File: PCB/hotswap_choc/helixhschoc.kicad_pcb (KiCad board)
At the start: 2 copper layers, 135.2 x 94 mm, 134 parts, among them J1 MJ-4PP-9, P1 CONN_01X01, P2 CONN_01X01, P3 OLED, P4 LED, SW1 SW_PUSH, SW10 SW_PUSH, SW11 SW_PUSH, SW12 SW_PUSH, SW13 SW_PUSH, SW14 SW_PUSH, SW15 SW_PUSH, SW16 SW_PUSH, SW17 SW_PUSH, SW18 SW_PUSH, SW19 SW_PUSH, SW2 SW_PUSH, SW20 SW_PUSH, SW21 SW_PUSH, SW22 SW_PUSH, SW23 SW_PUSH, SW24 SW_PUSH, SW25 SW_PUSH, SW26 SW_PUSH, SW27 SW_PUSH, SW28 SW_PUSH, SW29 SW_PUSH, SW3 SW_PUSH, SW30 SW_PUSH, SW31 SW_PUSH, SW32 SW_PUSH, SW33 Reset, SW4 SW_PUSH, SW5 SW_PUSH, SW6 SW_PUSH, SW7 SW_PUSH, SW8 SW_PUSH, SW9 SW_PUSH, U1 ProMicro, U10 SK6812mini, U11 SK6812mini, U12 SK6812mini, U13 SK6812mini, U14 SK6812mini, U15 SK6812mini, U16 SK6812mini, U17 SK6812mini, U18 SK6812mini, U19 SK6812mini, U2 SK6812mini, U20 SK6812mini, U21 SK6812mini, U22 SK6812mini, U23 SK6812mini, U24 SK6812mini, U25 SK6812mini, U26 SK6812mini, U27 SK6812mini, U28 SK6812mini, U29 SK6812mini, U3 SK6812mini, U30 SK6812mini, U31 SK6812mini, U32 SK6812mini, U33 SK6812mini, U4 SK6812mini, U5 SK6812mini, U6 SK6812mini, U7 SK6812mini, U8 SK6812mini, U9 SK6812mini

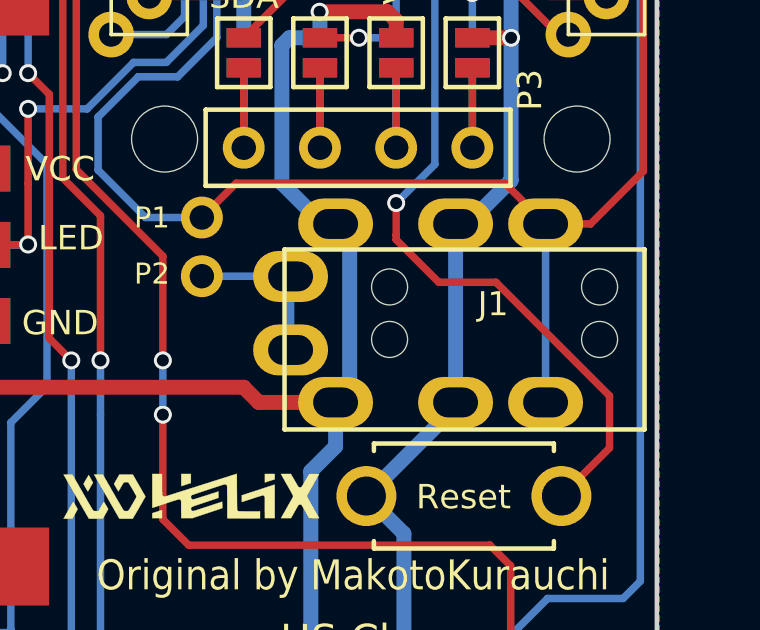
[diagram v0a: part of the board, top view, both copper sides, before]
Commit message: PCB WIP
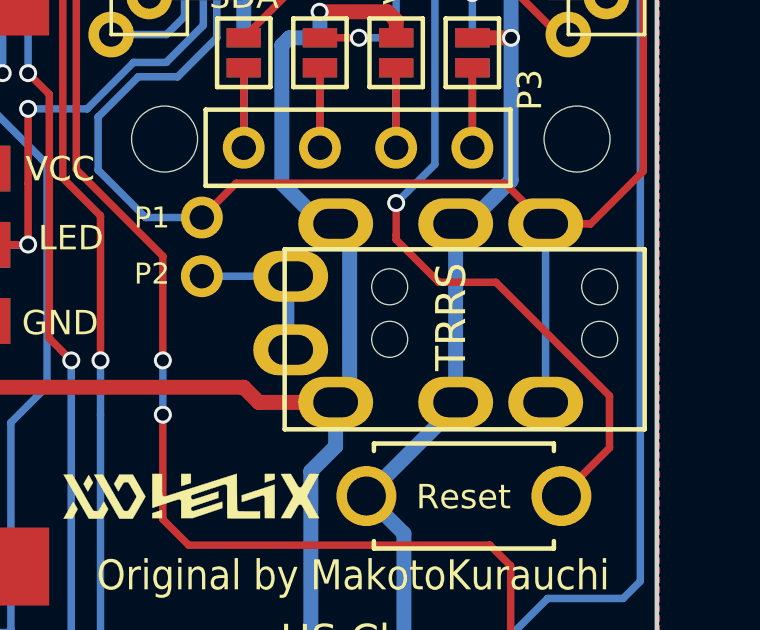
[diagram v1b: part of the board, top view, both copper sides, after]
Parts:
- J1: footprint MYLIB_REV:MJ-4PP-9_rev2 -> Random-keyboard-parts:MJ-4PP-9

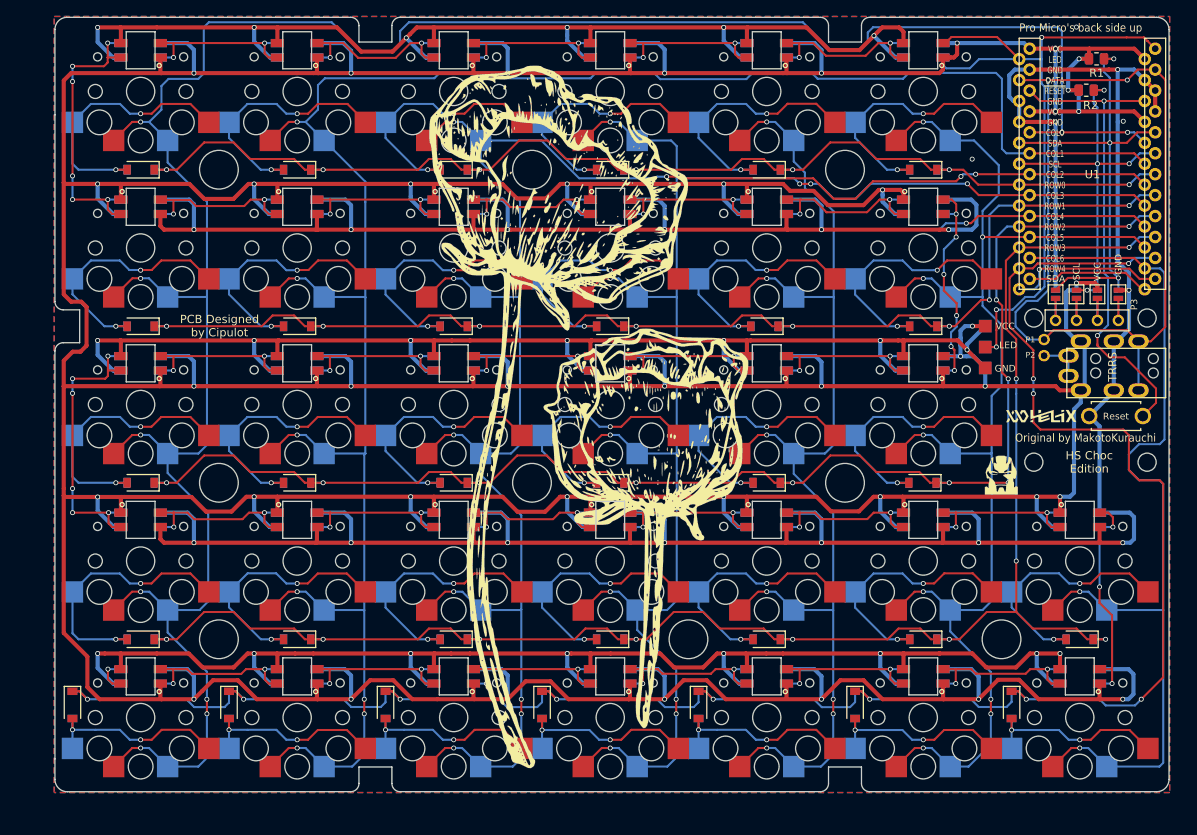
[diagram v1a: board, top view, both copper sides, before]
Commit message: PCB WIP
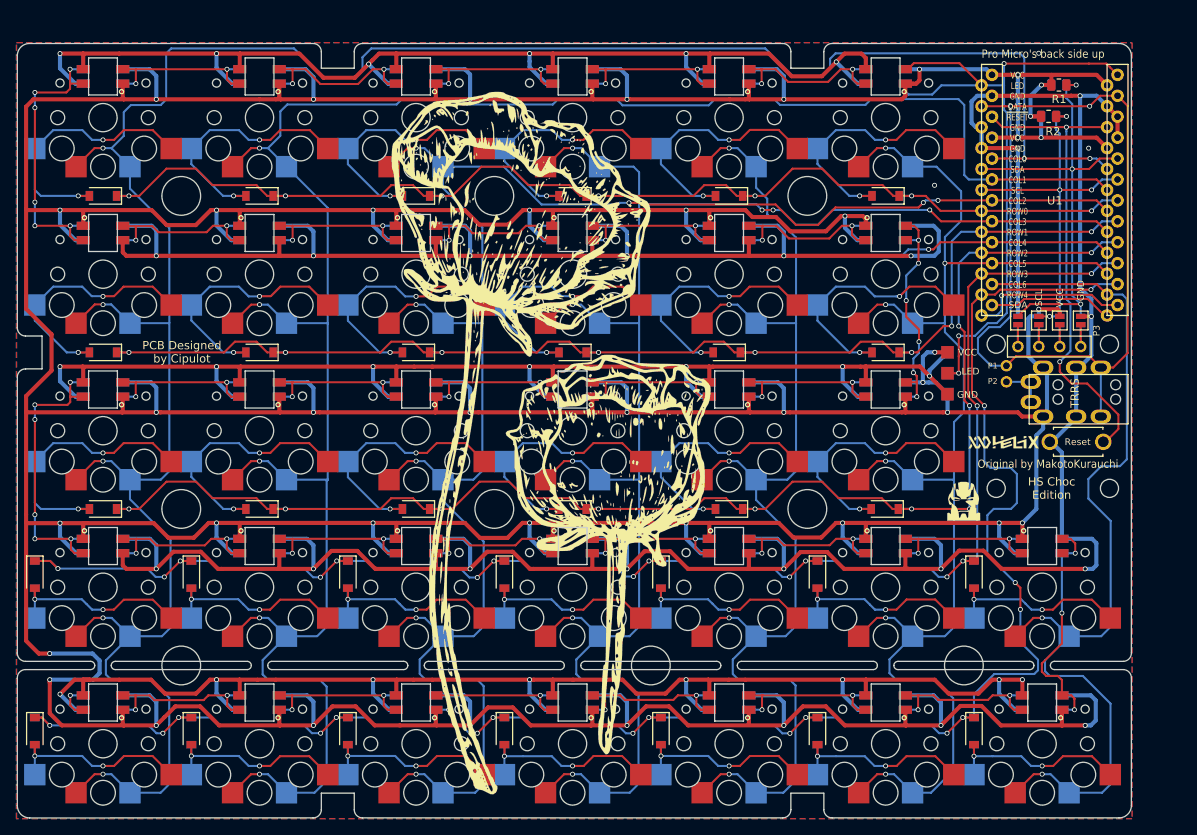
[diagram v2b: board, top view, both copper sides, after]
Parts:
- removed the G*** at (196.5, 99.5) (x2)
- removed the G*** at (201.3, 92.4) (x2)
- removed the R1 at (208.0, 49.0) (x2)
- removed the R2 at (206.8, 52.8) (x2)
- added G***: Helix_logo_small, Logos:Helix_logo_small, B.Cu at (196.8, 95.6)
- added G***: LOGO, Logos:IronMan_small, B.Cu at (191.9, 102.7)
- added G***: Helix_logo_small, Logos:Helix_logo_small, F.Cu at (196.8, 95.6)
- added G***: LOGO, Logos:IronMan_small, F.Cu at (191.9, 102.7)
- added R1: 10k, Resistor_SMD:R_0805_2012Metric, F.Cu at (203.5, 52.2)
- added R1: 10k, Resistor_SMD:R_0805_2012Metric, B.Cu at (203.4, 52.2)
- added R2: 10k, Resistor_SMD:R_0805_2012Metric, B.Cu at (202.2, 56.0)
- added R2: 10k, Resistor_SMD:R_0805_2012Metric, F.Cu at (202.2, 56.0)
- SW33: footprint MYLIB:SW_3.5x6.0_TH -> Random-keyboard-parts:SW_3.5x6.0_TH
- U10, U11, U12, U13, U14, U15, U16, U17, U18, U19, U20, U21, U22, U23, U24, U25, U26, U27, U28, U29, U3, U30, U31, U32, U33, U4, U5, U6, U7, U8, U9: footprint MYLIB_REV:SK6812MINI_rev -> LED_WS_SK:SK6812MINI_rev
- U2: footprint JMG:SK6812MINI_rev -> LED_WS_SK:SK6812MINI_rev
- moved D24 15.1 mm to (174.2, 111.6), turned to 270 degrees
- moved D19 15.1 mm to (79.2, 111.6), turned to 270 degrees
- moved D20 15.1 mm to (98.2, 111.6), turned to 270 degrees
- moved D21 15.1 mm to (117.2, 111.6), turned to 270 degrees
- moved D22 15.1 mm to (136.2, 111.6), turned to 270 degrees
- moved D23 15.1 mm to (155.2, 111.6), turned to 270 degrees
- moved D25 15.0 mm to (193.2, 111.6), turned to 270 degrees
- moved J1 5.57 mm to (211.9, 90.4)
- moved G*** 5.57 mm to (142.2, 95.4)
- moved D11 5.57 mm to (163.2, 84.7)
- moved D18 5.57 mm to (182.3, 103.7)
- moved G*** 5.57 mm to (133.8, 92.4)
- moved H11 5.57 mm to (208.7, 83.7)
- moved JP11 5.57 mm to (198.5, 80.8)
- moved JP7 5.57 mm to (198.5, 80.8)
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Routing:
- net row4: track 246.2 -> 218.2 mm, vias 11 -> 17
- net row3: track 199.9 -> 188.3 mm, vias 10 -> 15
- net VCC: track 1047.3 -> 1057.6 mm, vias 41 -> 43
- net Net-(D19-Pad2): track 32.7 -> 23.5 mm
- net GND: track 919.6 -> 928.5 mm, vias 40 -> 37
- net Net-(D24-Pad2): track 31.1 -> 23.5 mm
- net Net-(D20-Pad2): track 31.0 -> 23.5 mm
- net Net-(D21-Pad2): track 31.0 -> 23.5 mm
- net Net-(D22-Pad2): track 31.0 -> 23.5 mm
- net Net-(D25-Pad2): track 31.0 -> 23.5 mm
- net Net-(D23-Pad2): track 31.0 -> 23.5 mm
- net col1: track 256.5 -> 263.9 mm, vias 7 -> 5
- net col2: track 225.7 -> 233.1 mm, vias 10 -> 8
- net col4: track 179.2 -> 186.5 mm, vias 8 -> 6
- net col0: track 296.4 -> 301.6 mm, vias 9 -> 7
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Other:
- outline, holes or cut-outs redrawn

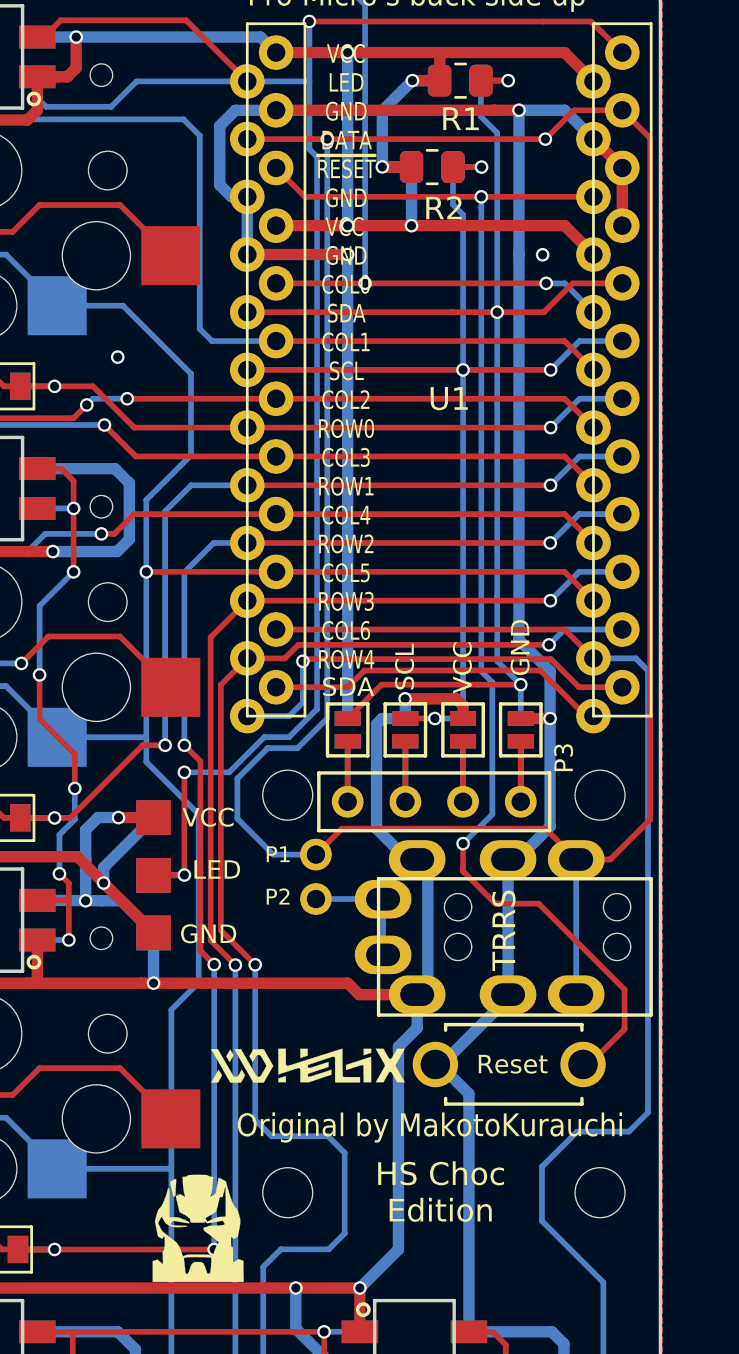
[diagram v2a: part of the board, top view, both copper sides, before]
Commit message: Pcb update
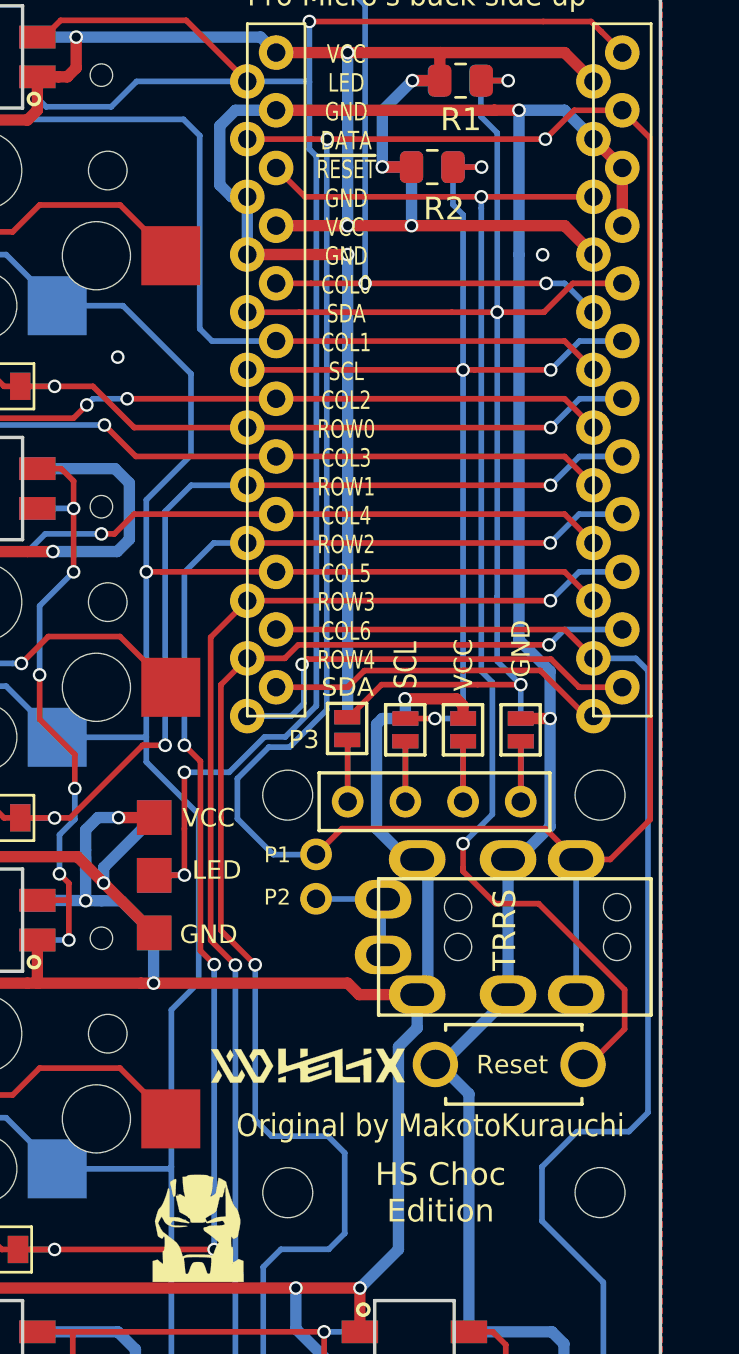
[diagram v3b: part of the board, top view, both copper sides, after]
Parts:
- GND: renamed from JP11; footprint MYLIB:Jumper -> Random-keyboard-parts:Jumper_Small
- GND: renamed from JP4; footprint MYLIB:Jumper -> Random-keyboard-parts:Jumper_Small
- H10, H11, H12, H13: footprint JMG:HOLE_M2 -> Random-keyboard-parts:HOLE_M2
- P1, P2: footprint MYLIB:1PIN_0.1 -> Random-keyboard-parts:Pin_Small
- P3: footprint MYLIB:MY_SIL-4 -> Random-keyboard-parts:OLED_Small
- P4: footprint MYLIB_REV:StripLED_rev -> Random-keyboard-parts:LED_Strip_Pad
- SCL: renamed from JP9; footprint MYLIB:Jumper -> Random-keyboard-parts:Jumper_Small
- SCL: renamed from JP6; footprint MYLIB:Jumper -> Random-keyboard-parts:Jumper_Small
- SDA: renamed from JP8; footprint MYLIB:Jumper -> Random-keyboard-parts:Jumper_Small
- SDA: renamed from JP7; footprint MYLIB:Jumper -> Random-keyboard-parts:Jumper_Small
- VCC: renamed from JP10; footprint MYLIB:Jumper -> Random-keyboard-parts:Jumper_Small
- VCC: renamed from JP5; footprint MYLIB:Jumper -> Random-keyboard-parts:Jumper_Small
- moved P3 3.77 mm to (202.3, 84.0), turned to 0 degrees
- moved P4 2.53 mm to (189.9, 87.2)
- moved H13 1.42 mm to (195.9, 101.2)
- moved H10 1.42 mm to (209.6, 101.2)
- moved H12 1.42 mm to (195.9, 83.7)
- moved H11 0.91 mm to (209.6, 83.7)
- moved VCC 0.06 mm to (203.6, 80.9), turned to 0 degrees
- moved SDA 0.06 mm to (206.1, 80.9), turned to 180 degrees
- moved GND 0.06 mm to (206.1, 80.9), turned to 0 degrees
- moved SCL 0.06 mm to (201.1, 80.9), turned to 0 degrees
- moved SCL 0.06 mm to (203.6, 80.9), turned to 180 degrees
- moved VCC 0.06 mm to (201.0, 80.9), turned to 180 degrees
- turned GND to 180 degrees
- turned SDA to 0 degrees
